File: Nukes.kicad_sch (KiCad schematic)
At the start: 25 parts, among them J6 Screw_Terminal_01x08, J7 Conn_01x05_Male, Q2 NCV8415STT1G, Q3 NCV8415STT1G, Q4 NCV8415STT1G, Q5 NCV8415STT1G, U3 LTV-247, U4 PCA9534RGVR, U5 PCA9685BS

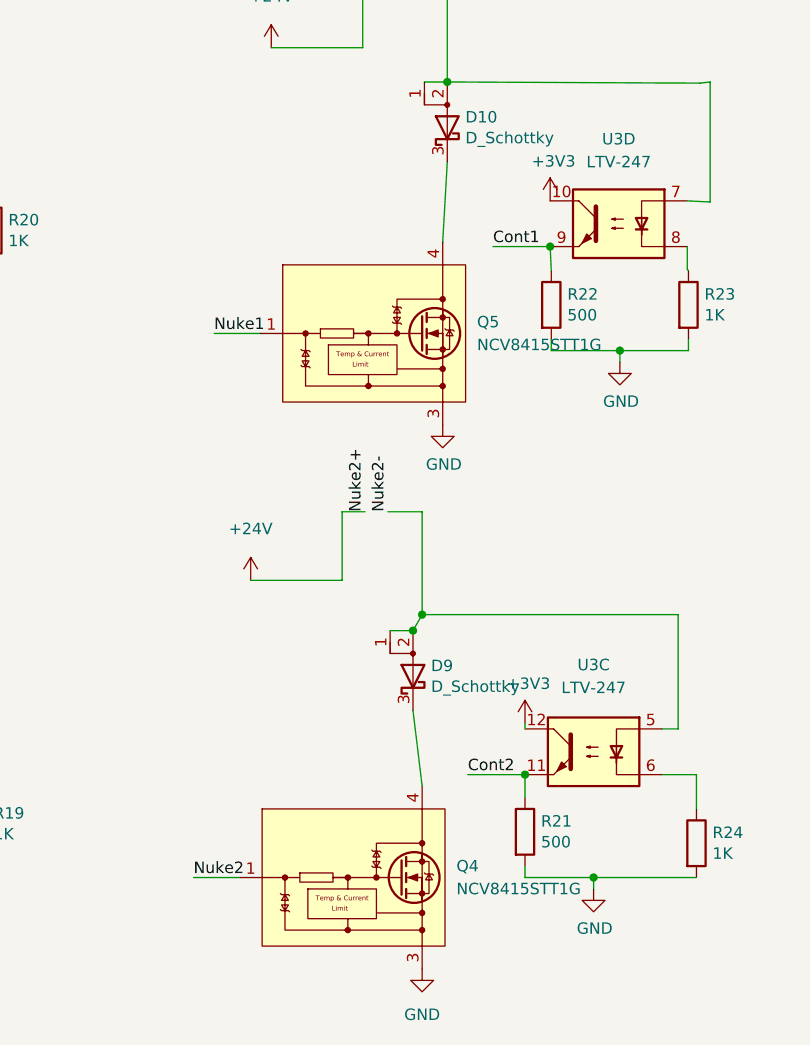
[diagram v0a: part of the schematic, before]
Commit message: update
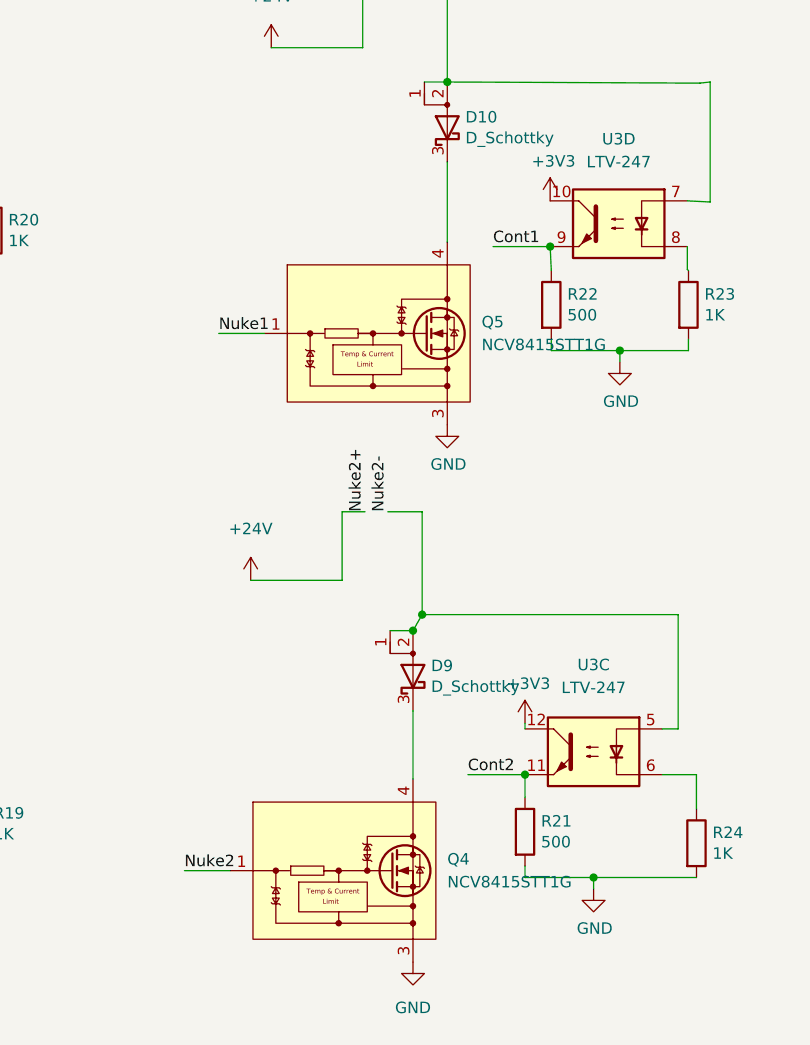
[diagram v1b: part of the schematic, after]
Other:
- moved on the sheet: Q4, Q5
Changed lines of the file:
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@@
     (stroke (width 0) (type default))
   )
-  (wire (pts (xy 91.186 181.102) (xy 96.266 181.102))
+  (wire (pts (xy 90.17 180.34) (xy 95.25 180.34))
     (stroke (width 0) (type default))
   )
@@
     (stroke (width 0) (type default))
   )
-  (wire (pts (xy 98.552 120.65) (xy 93.472 120.65))
+  (wire (pts (xy 99.06 120.65) (xy 93.98 120.65))
     (stroke (width 0) (type default))
   )
@@
     (stroke (width 0) (type default))
   )
-  (wire (pts (xy 115.57 162.56) (xy 116.586 170.942))
+  (wire (pts (xy 115.57 162.56) (xy 115.57 170.18))
     (stroke (width 0) (type default))
   )
@@
     (stroke (width 0) (type default))
   )
-  (wire (pts (xy 119.38 101.6) (xy 118.872 110.49))
+  (wire (pts (xy 119.38 101.6) (xy 119.38 110.49))
     (stroke (width 0) (type default))
   )
@@
     (effects (font (size 1.27 1.27)) (justify left bottom))
   )
-  (label "Nuke1" (at 93.472 120.65 0) (fields_autoplaced)
+  (label "Nuke1" (at 93.98 120.65 0) (fields_autoplaced)
     (effects (font (size 1.27 1.27)) (justify left bottom))
   )
@@
     (effects (font (size 1.27 1.27)) (justify left bottom))
   )
-  (label "Nuke2" (at 91.186 181.102 0) (fields_autoplaced)
+  (label "Nuke2" (at 90.17 180.34 0) (fields_autoplaced)
     (effects (font (size 1.27 1.27)) (justify left bottom))
   )
@@
     )
   )
-  (symbol (lib_id "power:GND") (at 116.586 191.262 0) (unit 1)
-    (in_bom yes) (on_board yes) (dnp no) (fields_autoplaced)
-    (property "Reference" "#PWR056" (at 116.586 197.612 0)
-      (effects (font (size 1.27 1.27)) hide)
-    )
-    (property "Value" "GND" (at 116.586 196.342 0)
-      (effects (font (size 1.27 1.27)))
-    )
-    (property "Footprint" "" (at 116.586 191.262 0)
-      (effects (font (size 1.27 1.27)) hide)
-    )
-    (property "Datasheet" "" (at 116.586 191.262 0)
+  (symbol (lib_id "power:GND") (at 115.57 190.5 0) (unit 1)
+    (in_bom yes) (on_board yes) (dnp no) (fields_autoplaced)
+    (property "Reference" "#PWR056" (at 115.57 196.85 0)
+      (effects (font (size 1.27 1.27)) hide)
+    )
+    (property "Value" "GND" (at 115.57 195.58 0)
+      (effects (font (size 1.27 1.27)))
+    )
+    (property "Footprint" "" (at 115.57 190.5 0)
+      (effects (font (size 1.27 1.27)) hide)
+    )
+    (property "Datasheet" "" (at 115.57 190.5 0)
       (effects (font (size 1.27 1.27)) hide)
     )
@@
     )
   )
-  (symbol (lib_id "Driver_FET:NCV8402xST") (at 111.252 120.65 0) (unit 1)
-    (in_bom yes) (on_board yes) (dnp no) (fields_autoplaced)
-    (property "Reference" "Q5" (at 122.682 119.3799 0)
-      (effects (font (size 1.27 1.27)) (justify left))
-    )
-    (property "Value" "NCV8415STT1G" (at 122.682 121.9199 0)
-      (effects (font (size 1.27 1.27)) (justify left))
-    )
-    (property "Footprint" "Package_TO_SOT_SMD:SOT-223" (at 111.252 127.762 0)
-      (effects (font (size 1.27 1.27)) hide)
-    )
-    (property "Datasheet" "https://www.onsemi.com/pub/Collateral/NCV8402-D.PDF" (at 118.872 120.65 0)
+  (symbol (lib_id "Driver_FET:NCV8402xST") (at 111.76 120.65 0) (unit 1)
+    (in_bom yes) (on_board yes) (dnp no) (fields_autoplaced)
+    (property "Reference" "Q5" (at 123.19 119.3799 0)
+      (effects (font (size 1.27 1.27)) (justify left))
+    )
+    (property "Value" "NCV8415STT1G" (at 123.19 121.9199 0)
+      (effects (font (size 1.27 1.27)) (justify left))
+    )
+    (property "Footprint" "Package_TO_SOT_SMD:SOT-223" (at 111.76 127.762 0)
+      (effects (font (size 1.27 1.27)) hide)
+    )
+    (property "Datasheet" "https://www.onsemi.com/pub/Collateral/NCV8402-D.PDF" (at 119.38 120.65 0)
       (effects (font (size 1.27 1.27)) hide)
     )
@@
     )
   )
-  (symbol (lib_id "power:GND") (at 118.872 130.81 0) (unit 1)
-    (in_bom yes) (on_board yes) (dnp no)
-    (property "Reference" "#PWR057" (at 118.872 137.16 0)
-      (effects (font (size 1.27 1.27)) hide)
-    )
-    (property "Value" "GND" (at 118.999 135.2042 0)
-      (effects (font (size 1.27 1.27)))
-    )
-    (property "Footprint" "" (at 118.872 130.81 0)
-      (effects (font (size 1.27 1.27)) hide)
-    )
-    (property "Datasheet" "" (at 118.872 130.81 0)
+  (symbol (lib_id "power:GND") (at 119.38 130.81 0) (unit 1)
+    (in_bom yes) (on_board yes) (dnp no)
+    (property "Reference" "#PWR057" (at 119.38 137.16 0)
+      (effects (font (size 1.27 1.27)) hide)
+    )
+    (property "Value" "GND" (at 119.507 135.2042 0)
+      (effects (font (size 1.27 1.27)))
+    )
+    (property "Footprint" "" (at 119.38 130.81 0)
+      (effects (font (size 1.27 1.27)) hide)
+    )
+    (property "Datasheet" "" (at 119.38 130.81 0)
       (effects (font (size 1.27 1.27)) hide)
     )
@@
     )
   )
-  (symbol (lib_id "Driver_FET:NCV8402xST") (at 108.966 181.102 0) (unit 1)
-    (in_bom yes) (on_board yes) (dnp no) (fields_autoplaced)
-    (property "Reference" "Q4" (at 120.396 179.8319 0)
-      (effects (font (size 1.27 1.27)) (justify left))
-    )
-    (property "Value" "NCV8415STT1G" (at 120.396 182.3719 0)
-      (effects (font (size 1.27 1.27)) (justify left))
-    )
-    (property "Footprint" "Package_TO_SOT_SMD:SOT-223" (at 108.966 188.214 0)
-      (effects (font (size 1.27 1.27)) hide)
-    )
-    (property "Datasheet" "https://www.onsemi.com/pub/Collateral/NCV8402-D.PDF" (at 116.586 181.102 0)
-      (effects (font (size 1.27 1.27)) hide)
-    )
+  (symbol (lib_id "Driver_FET:NCV8402xST") (at 107.95 180.34 0) (unit 1)
+    (in_bom yes) (on_board yes) (dnp no) (fields_autoplaced)
+    (property "Reference" "Q4" (at 119.38 179.0699 0)
+      (effects (font (size 1.27 1.27)) (justify left))
+    )
+    (property "Value" "NCV8415STT1G" (at 119.38 181.6099 0)
+      (effects (font (size 1.27 1.27)) (justify left))
+    )
+    (property "Footprint" "Package_TO_SOT_SMD:SOT-223" (at 107.95 187.452 0)
+      (effects (font (size 1.27 1.27)) hide)
+    )
+    (property "Datasheet" "https://www.onsemi.com/pub/Collateral/NCV8402-D.PDF" (at 115.57 180.34 0)
+      (effects (font (size 1.27 1.27)) hide)
+    )
